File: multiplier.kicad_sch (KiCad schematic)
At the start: 4 parts, among them U31 4081, U32 4081, U33 4081, U34 4069

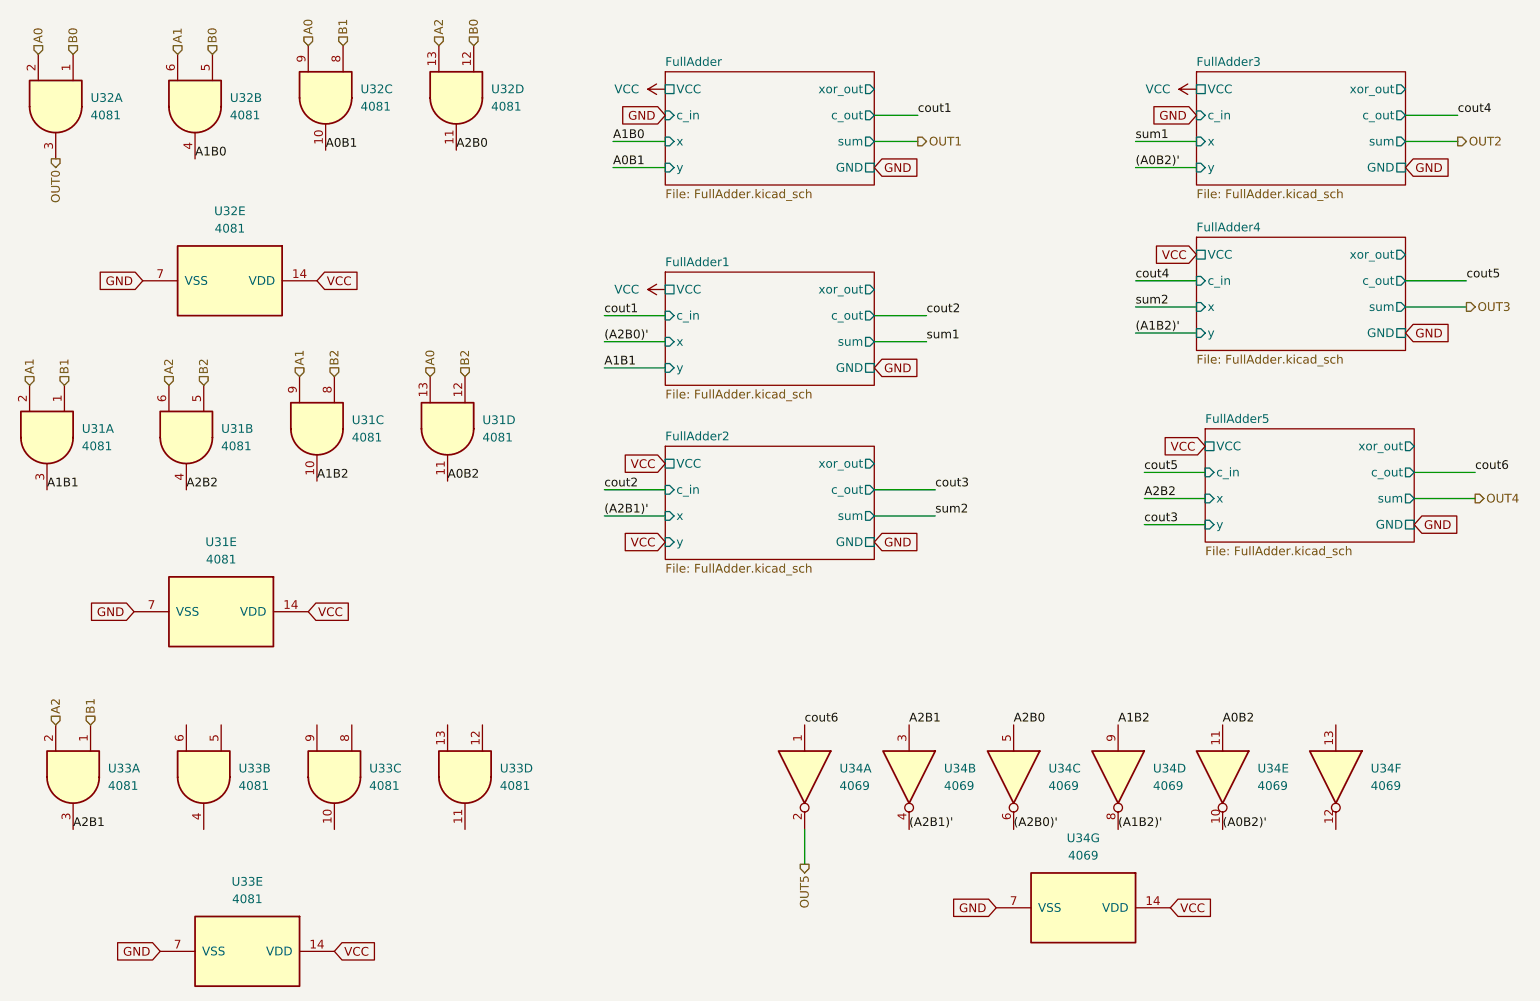
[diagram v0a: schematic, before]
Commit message: Add files via upload
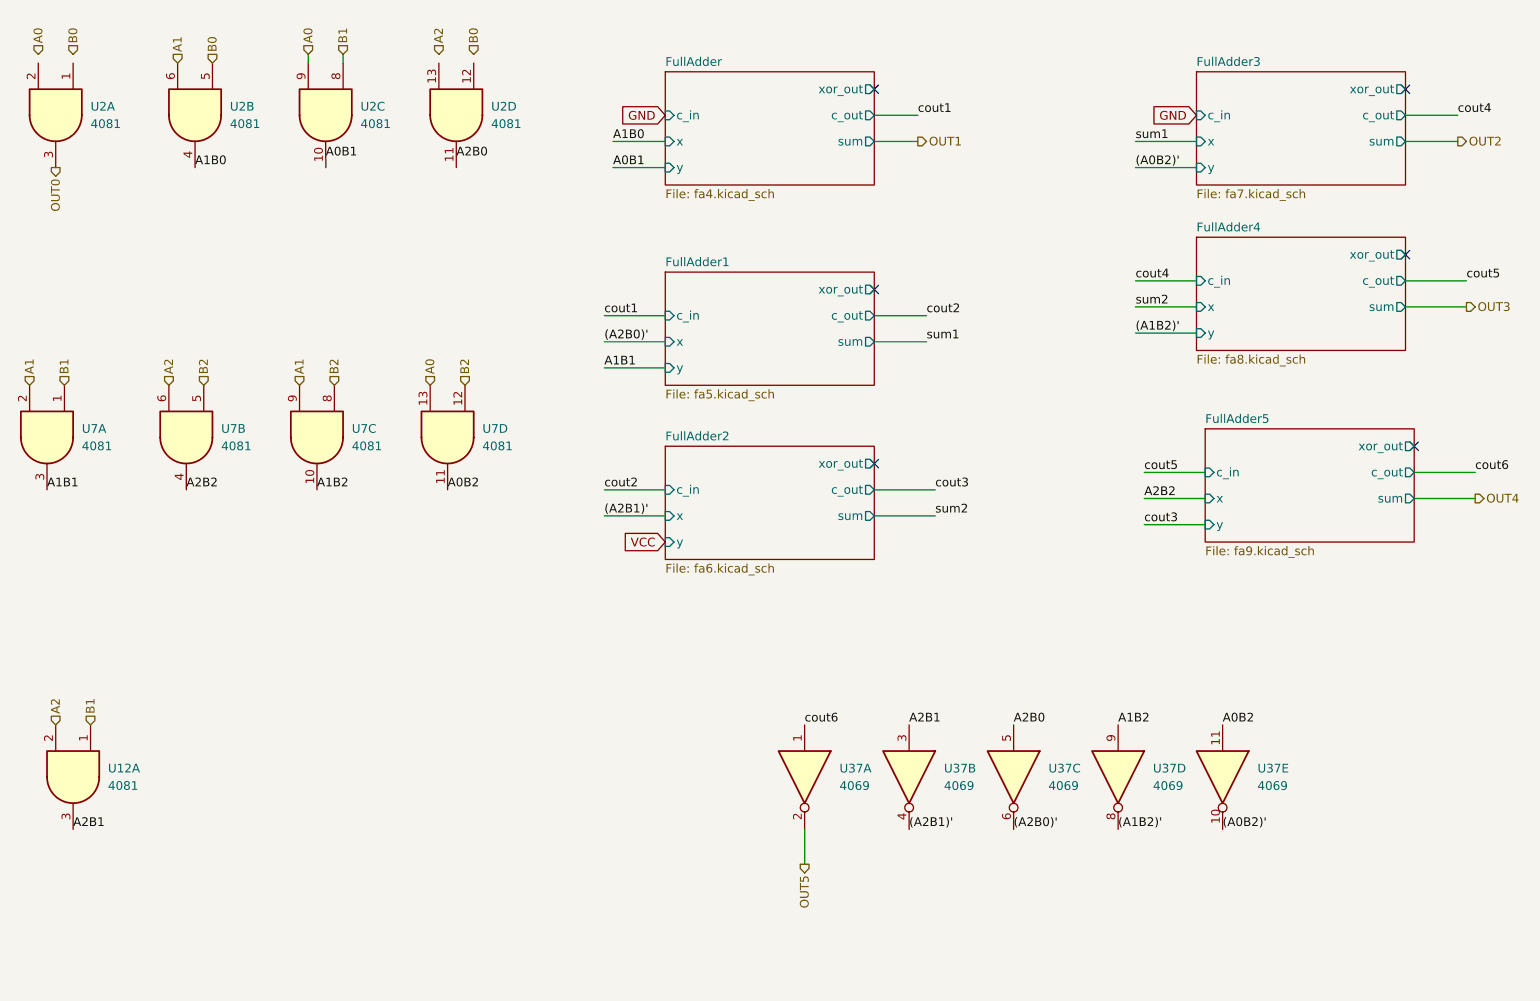
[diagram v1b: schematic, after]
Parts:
- removed U31, U32, U33: 4081, Package_DIP:CERDIP-14_W7.62mm_SideBrazed_LongPads_Socket, symbol 4xxx:4081
- removed U34: 4069, Package_DIP:CERDIP-14_W7.62mm_SideBrazed_LongPads_Socket, symbol 4xxx:4069
- added U12, U2, U7: 4081, Package_DIP:CERDIP-14_W7.62mm_SideBrazed_LongPads_Socket, symbol 4xxx:4081
- added U37: 4069, Package_DIP:CERDIP-14_W7.62mm_SideBrazed_LongPads_Socket, symbol 4xxx:4069
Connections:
- net (A0B2)': now also U37.10
- net (A1B2)': now also U37.8
- net (A2B0)': now also U37.6
- net (A2B1)': now also U37.4
- net A0: now also U2.9, U7.13
- net A0B1: now also U2.10
- net A0B2: now also U37.11, U7.11
- net A1: now also U2.6, U7.2, U7.9
- net A1B0: now also U2.4
- net A1B1: now also U7.3
- net A1B2: now also U37.9, U7.10
- net A2: now also U12.2, U7.6
- net A2B0: now also U37.5
- net A2B1: now also U12.3, U37.3
- net A2B2: now also U7.4
- net B0: now also U2.5
- net B1: now also U12.1, U2.8, U7.1
- net B2: now also U7.12, U7.5, U7.8
- net OUT0: now also U2.3
- net OUT5: now also U37.2
- net cout6: now also U37.1
- no-connect marks 0 -> 6
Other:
- sheet FullAdder: file FullAdder.kicad_sch -> fa4.kicad_sch
- sheet FullAdder ports: added none; removed GND, VCC
- sheet FullAdder1: file FullAdder.kicad_sch -> fa5.kicad_sch
- sheet FullAdder1 ports: added none; removed GND, VCC
- sheet FullAdder2: file FullAdder.kicad_sch -> fa6.kicad_sch
- sheet FullAdder2 ports: added none; removed GND, VCC
- sheet FullAdder3: file FullAdder.kicad_sch -> fa7.kicad_sch
- sheet FullAdder3 ports: added none; removed GND, VCC
- sheet FullAdder4: file FullAdder.kicad_sch -> fa8.kicad_sch
- sheet FullAdder4 ports: added none; removed GND, VCC
- sheet FullAdder5: file FullAdder.kicad_sch -> fa9.kicad_sch
- sheet FullAdder5 ports: added none; removed GND, VCC
